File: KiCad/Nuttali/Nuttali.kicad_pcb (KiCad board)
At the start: 2 copper layers, 52.7 x 101.7 mm, 85 parts, among them J1 SWD, J2 B4B-XH-A, SW1 SW_DPST_x2, SW10 SW_Push, SW2 RND 210-00662, SW3 SW_Push, SW4 SW_Push, SW5 SW_Push, SW6 SW_Push, SW7 SW_Push, SW8 Rotary_Encoder, U1 STM32F411RETx, U2 PMW3389, U3 USBLC6-2P6, U4 AP131-15, U5 AP1117-15, Y1 16Mhz

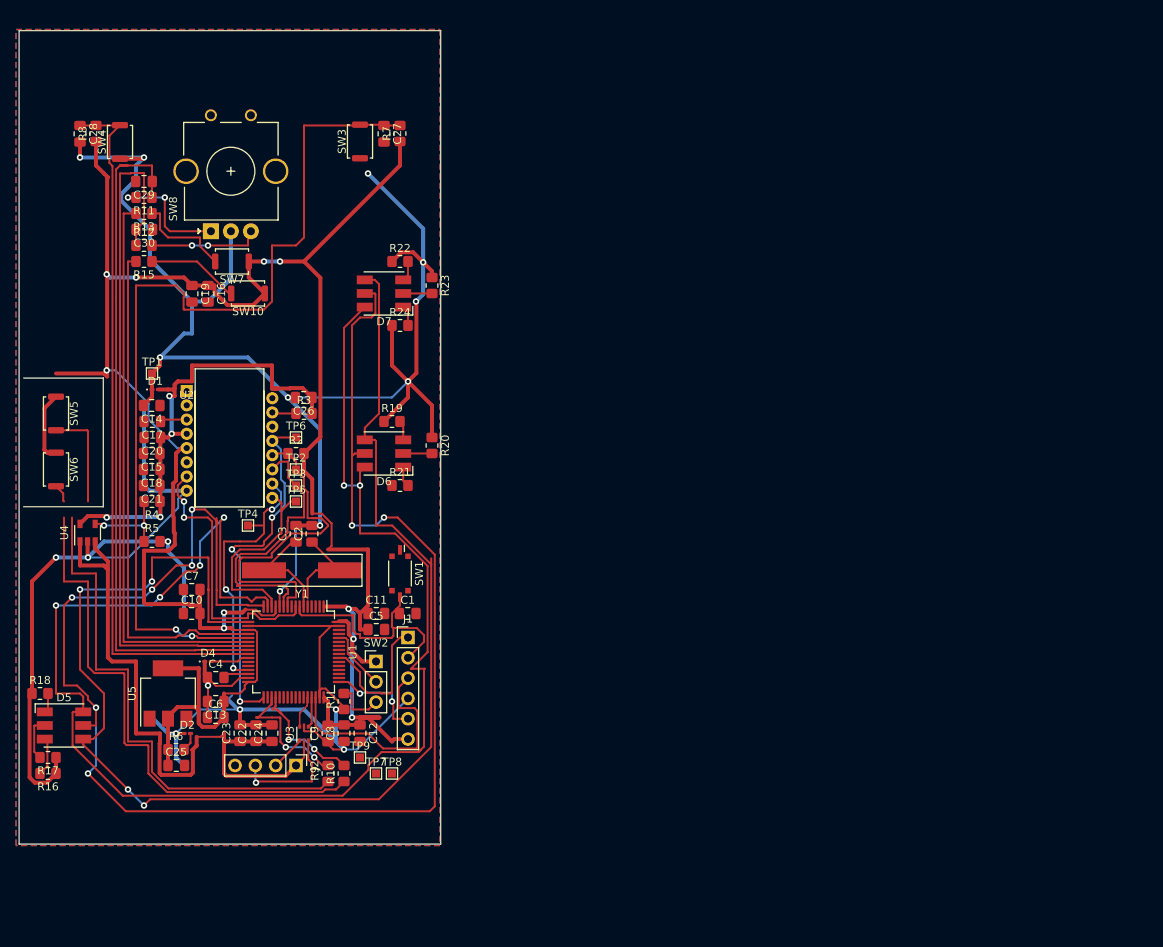
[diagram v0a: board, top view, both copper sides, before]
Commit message: Working on the new pcb
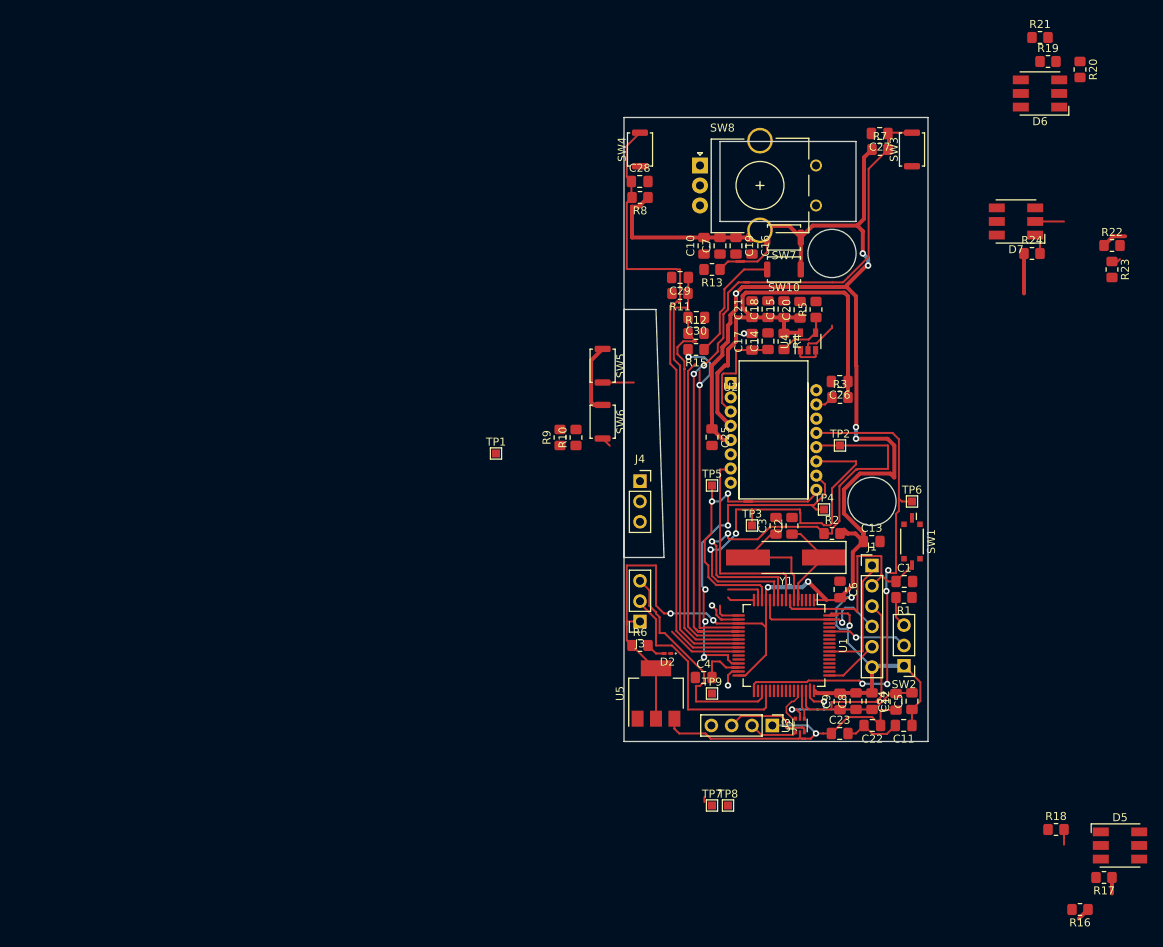
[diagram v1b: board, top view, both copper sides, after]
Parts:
- removed D1, D4: LED, LED_SMD:LED_0201_0603Metric_Pad0.64x0.40mm_HandSolder
- added J3: Conn_01x03_Male, Connector_PinSocket_2.54mm:PinSocket_1x03_P2.54mm_Vertical, F.Cu at (192.0, 117.3)
- added J4: Conn_01x03_Male, Connector_PinSocket_2.54mm:PinSocket_1x03_P2.54mm_Vertical, F.Cu at (192.0, 99.8)
- moved D5 132.8 mm to (252.0, 145.3)
- moved R17 132.8 mm to (250.0, 149.3)
- moved R16 130.1 mm to (247.0, 153.3)
- moved R18 128.1 mm to (244.0, 143.3)
- moved R21 97.7 mm to (242.0, 44.3)
- moved R20 93.6 mm to (247.0, 48.3)
- moved D6 93.5 mm to (242.0, 51.3)
- moved R19 93.5 mm to (243.0, 47.3)
- moved U4 93.2 mm to (213.0, 82.3)
- moved R22 89.0 mm to (251.0, 70.3)
- moved R5 87.9 mm to (214.0, 78.3), turned to 90 degrees
- moved R23 85.0 mm to (251.0, 73.3)
- moved C13 84.4 mm to (221.0, 107.3), turned to 0 degrees
- moved C20 82.5 mm to (212.0, 78.4), turned to 90 degrees
- moved R4 81.5 mm to (210.0, 82.3), turned to 270 degrees
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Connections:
- R10 pad 2: SideBack -> Net-(J4-Pad2)
- R9 pad 2: SideFront -> Net-(J4-Pad3)
- SW5 pad 1: VDDIO_3.3V -> Net-(J4-Pad1)
- SW6 pad 1: VDDIO_3.3V -> Net-(J4-Pad1)
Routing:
- net GND: track 396.6 -> 74.1 mm, vias 18 -> 6
- net G_LED: track 199.4 -> 3.38 mm, vias 8 -> 0
- net R_LED: track 186.2 -> 5.65 mm, vias 6 -> 0
- net B_LED: track 171.9 -> 3.43 mm, vias 4 -> 0
- net Net-(R9-Pad1): track 78.9 -> 3.90 mm
- net Net-(R10-Pad1): track 70.1 -> 1.27 mm
- net VDDIO_3.3V: track 314.2 -> 268.6 mm, vias 10 -> 11
- net WheelB: track 87.5 -> 49.0 mm
- net +5V: track 80.1 -> 43.3 mm, vias 0 -> 1
- net WheelA: track 86.4 -> 54.4 mm
- net WheelButton: track 70.7 -> 40.0 mm
- net RightB: track 114.9 -> 90.9 mm
- net Turbo: track 63.6 -> 44.4 mm, vias 0 -> 2
- net NCS: track 44.7 -> 62.6 mm, vias 3 -> 4
- net MISO: track 41.6 -> 58.0 mm, vias 0 -> 2
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- removed copper zone on B.Cu, net GND
- removed copper zone on F.Cu, net GND
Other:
- board size 52.7 x 101.7 mm -> 38 x 78 mm
